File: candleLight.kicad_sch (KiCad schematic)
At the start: 42 parts, among them J1 USB_C_Receptacle_USB2.0, J2 Conn_Phoenix, J3 Conn_SWD, J4 Conn_USART1, J5 Conn_BOOT0, SW1 MST22D18G2 125, U1 STM32F072C8Tx, U2 AMS1117-3.3, U3 TJA1051TK-3, Y1 8MHz

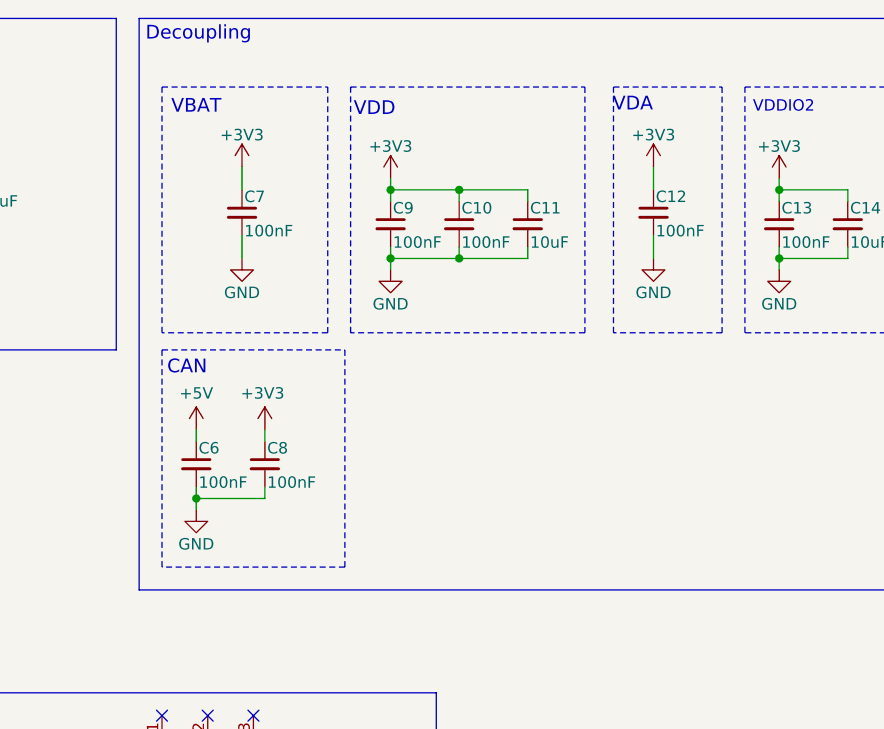
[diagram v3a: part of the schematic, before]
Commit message: update silkscreen
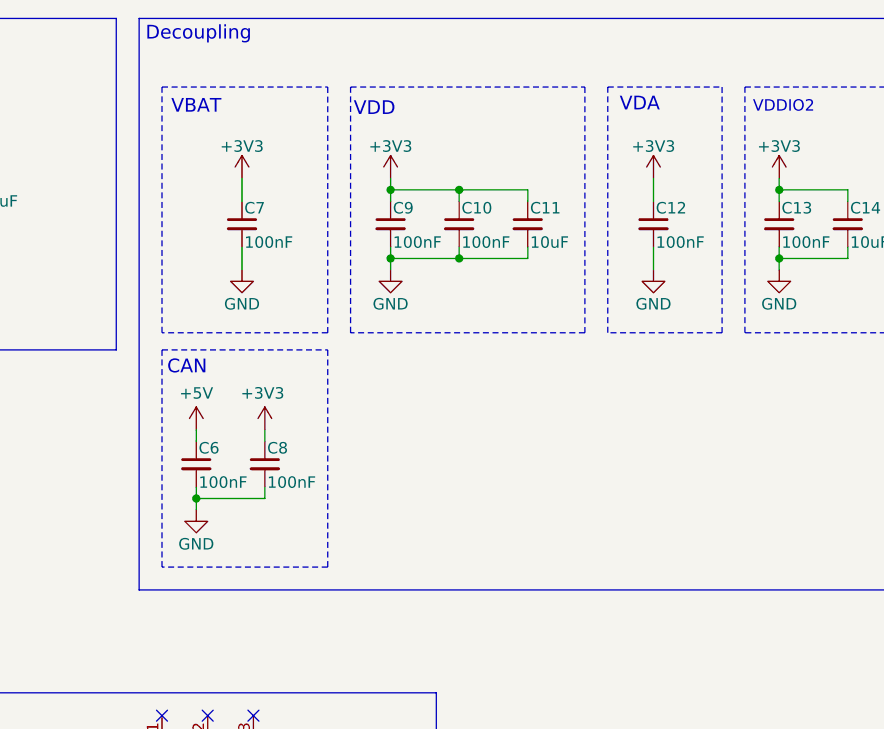
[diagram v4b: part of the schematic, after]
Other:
- moved on the sheet: C12, C7
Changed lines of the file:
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@@
 	)
 	(rectangle
-		(start 247.015 21.59)
+		(start 246.38 21.59)
 		(end 259.08 48.895)
 		(stroke
@@
 	(rectangle
 		(start 196.85 50.8)
-		(end 217.17 74.93)
+		(end 215.265 74.93)
 		(stroke
 			(width 0)
@@
 	(text "VDA"
 		(exclude_from_sim no)
-		(at 249.174 23.622 0)
+		(at 249.936 23.622 0)
 		(effects
 			(font
@@
 	(wire
 		(pts
-			(xy 251.46 38.1) (xy 251.46 40.64)
+			(xy 251.46 39.37) (xy 251.46 41.91)
 		)
 		(stroke
@@
 	(wire
 		(pts
-			(xy 205.74 38.1) (xy 205.74 40.64)
+			(xy 205.74 39.37) (xy 205.74 41.91)
 		)
 		(stroke
@@
 	(wire
 		(pts
-			(xy 205.74 30.48) (xy 205.74 33.02)
+			(xy 205.74 31.75) (xy 205.74 34.29)
 		)
 		(stroke
@@
 	(wire
 		(pts
-			(xy 251.46 30.48) (xy 251.46 33.02)
+			(xy 251.46 31.75) (xy 251.46 34.29)
 		)
 		(stroke
@@
 		(lib_name "+3.3V_12")
 		(lib_id "candleLight-rescue:+3.3V")
-		(at 205.74 30.48 0)
+		(at 205.74 31.75 0)
 		(unit 1)
 		(exclude_from_sim no)
@@
 		(dnp no)
 		(property "Reference" "#PWR023"
-			(at 205.74 34.29 0)
+			(at 205.74 35.56 0)
 			(effects
 				(font
@@
 		)
 		(property "Value" "+3V3"
-			(at 205.74 26.924 0)
+			(at 205.74 28.194 0)
 			(effects
 				(font
@@
 		)
 		(property "Footprint" ""
-			(at 205.74 30.48 0)
+			(at 205.74 31.75 0)
 			(effects
 				(font
@@
 		)
 		(property "Datasheet" ""
-			(at 205.74 30.48 0)
+			(at 205.74 31.75 0)
 			(effects
 				(font
@@
 		)
 		(property "Description" ""
-			(at 205.74 30.48 0)
+			(at 205.74 31.75 0)
 			(effects
 				(font
@@
 	(symbol
 		(lib_id "power:GND")
-		(at 251.46 40.64 0)
+		(at 251.46 41.91 0)
 		(unit 1)
 		(exclude_from_sim no)
@@
 		(dnp no)
 		(property "Reference" "#PWR030"
-			(at 251.46 46.99 0)
+			(at 251.46 48.26 0)
 			(effects
 				(font
@@
 		)
 		(property "Value" "GND"
-			(at 251.46 44.45 0)
+			(at 251.46 45.72 0)
 			(effects
 				(font
@@
 		)
 		(property "Footprint" ""
-			(at 251.46 40.64 0)
+			(at 251.46 41.91 0)
 			(effects
 				(font
@@
 		)
 		(property "Datasheet" ""
-			(at 251.46 40.64 0)
+			(at 251.46 41.91 0)
 			(effects
 				(font
@@
 		)
 		(property "Description" "Power symbol creates a global label with name \"GND\" , ground"
-			(at 251.46 40.64 0)
+			(at 251.46 41.91 0)
 			(effects
 				(font
@@
 	(symbol
 		(lib_id "power:GND")
-		(at 205.74 40.64 0)
+		(at 205.74 41.91 0)
 		(unit 1)
 		(exclude_from_sim no)
@@
 		(dnp no)
 		(property "Reference" "#PWR024"
-			(at 205.74 46.99 0)
+			(at 205.74 48.26 0)
 			(effects
 				(font
@@
 		)
 		(property "Value" "GND"
-			(at 205.74 44.45 0)
+			(at 205.74 45.72 0)
 			(effects
 				(font
@@
 		)
 		(property "Footprint" ""
-			(at 205.74 40.64 0)
+			(at 205.74 41.91 0)
 			(effects
 				(font
@@
 		)
 		(property "Datasheet" ""
-			(at 205.74 40.64 0)
+			(at 205.74 41.91 0)
 			(effects
 				(font
@@
 		)
 		(property "Description" "Power symbol creates a global label with name \"GND\" , ground"
-			(at 205.74 40.64 0)
+			(at 205.74 41.91 0)
 			(effects
 				(font
@@
 	(symbol
 		(lib_id "Device:C_Small")
-		(at 251.46 35.56 0)
+		(at 251.46 36.83 0)
 		(unit 1)
 		(exclude_from_sim no)
@@
 		(dnp no)
 		(property "Reference" "C12"
-			(at 251.714 33.782 0)
+			(at 251.714 35.052 0)
 			(effects
 				(font
@@
 		)
 		(property "Value" "100nF"
-			(at 251.714 37.592 0)
+			(at 251.714 38.862 0)
 			(effects
 				(font
@@
 		)
 		(property "Footprint" "Capacitor_SMD:C_0603_1608Metric"
-			(at 251.46 35.56 0)
+			(at 251.46 36.83 0)
 			(effects
 				(font
@@
 		)
 		(property "Datasheet" "~"
-			(at 251.46 35.56 0)
+			(at 251.46 36.83 0)
 			(effects
 				(font
@@
 		)
 		(property "Description" "Unpolarized capacitor, small symbol"
-			(at 251.46 35.56 0)
+			(at 251.46 36.83 0)
 			(effects
 				(font
@@
 		)
 		(property "LCSC" "C14663"
-			(at 251.46 35.56 0)
+			(at 251.46 36.83 0)
 			(effects
 				(font
@@
 	(symbol
 		(lib_id "Device:C_Small")
-		(at 205.74 35.56 0)
+		(at 205.74 36.83 0)
 		(unit 1)
 		(exclude_from_sim no)
@@
 		(dnp no)
 		(property "Reference" "C7"
-			(at 205.994 33.782 0)
+			(at 205.994 35.052 0)
 			(effects
 				(font
@@
 		)
 		(property "Value" "100nF"
-			(at 205.994 37.592 0)
+			(at 205.994 38.862 0)
 			(effects
 				(font
@@
 		)
 		(property "Footprint" "Capacitor_SMD:C_0603_1608Metric"
-			(at 205.74 35.56 0)
+			(at 205.74 36.83 0)
 			(effects
 				(font
@@
 		)
 		(property "Datasheet" "~"
-			(at 205.74 35.56 0)
+			(at 205.74 36.83 0)
 			(effects
 				(font
@@
 		)
 		(property "Description" "Unpolarized capacitor, small symbol"
-			(at 205.74 35.56 0)
+			(at 205.74 36.83 0)
 			(effects
 				(font
@@
 		)
 		(property "LCSC" "C14663"
-			(at 205.74 35.56 0)
+			(at 205.74 36.83 0)
 			(effects
 				(font
@@
 		(lib_name "+3.3V_12")
 		(lib_id "candleLight-rescue:+3.3V")
-		(at 251.46 30.48 0)
+		(at 251.46 31.75 0)
 		(unit 1)
 		(exclude_from_sim no)
@@
 		(dnp no)
 		(property "Reference" "#PWR029"
-			(at 251.46 34.29 0)
+			(at 251.46 35.56 0)
 			(effects
 				(font
@@
 		)
 		(property "Value" "+3V3"
-			(at 251.46 26.924 0)
+			(at 251.46 28.194 0)
 			(effects
 				(font
@@
 		)
 		(property "Footprint" ""
-			(at 251.46 30.48 0)
+			(at 251.46 31.75 0)
 			(effects
 				(font
@@
 		)
 		(property "Datasheet" ""
-			(at 251.46 30.48 0)
+			(at 251.46 31.75 0)
 			(effects
 				(font
@@
 		)
 		(property "Description" ""
-			(at 251.46 30.48 0)
+			(at 251.46 31.75 0)
 			(effects
 				(font
